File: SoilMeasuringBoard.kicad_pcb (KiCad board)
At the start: 2 copper layers, 22.5 x 100 mm, 40 parts, among them J1 USB_B_Micro, J2 BATT_CONN, J3 Conn_01x07, Q1 Q_NMOS_GSD, Q2 DMP3099L-13, Q3 DMP3099L-13, U1 RFD77101, U2 MCP73811T-420I-OT, U3 TLV74130, U4 DS18B20U, U5 SST26VF016B

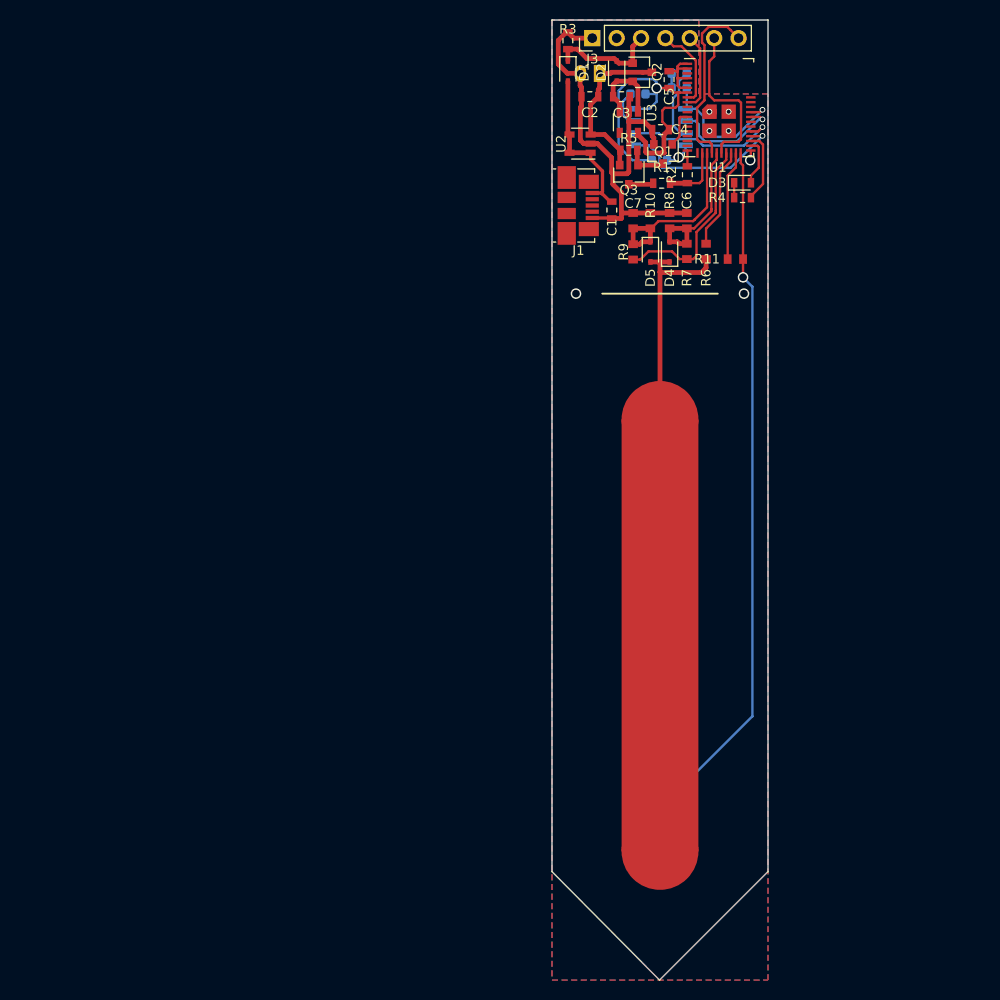
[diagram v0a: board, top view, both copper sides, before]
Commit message: final fixes
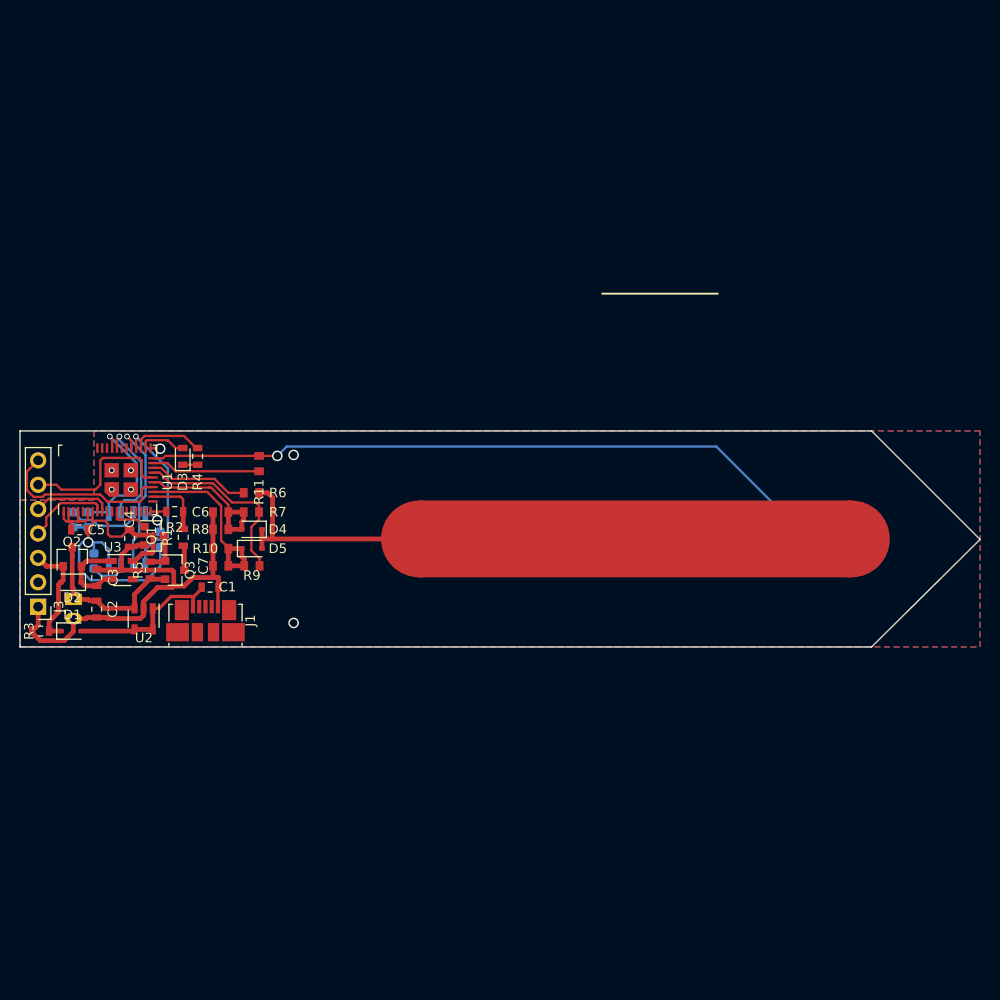
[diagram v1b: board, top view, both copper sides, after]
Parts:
- moved J3 82.7 mm to (84.1, 99.3), turned to 180 degrees
- moved R3 82.4 mm to (84.4, 101.8), turned to 180 degrees
- moved R13 78.4 mm to (87.8, 90.3), turned to 90 degrees
- moved D1 78.0 mm to (87.6, 101.8), turned to 0 degrees
- moved Q2 77.9 mm to (87.7, 94.1), turned to 90 degrees
- moved D2 77.9 mm to (87.6, 96.8), turned to 180 degrees
- moved J2 77.5 mm to (87.8, 98.5), turned to 270 degrees
- moved C5 77.3 mm to (88.4, 91.3), turned to 180 degrees
- moved R14 76.3 mm to (89.3, 90.3), turned to 90 degrees
- moved R12 74.7 mm to (89.9, 94.6), turned to 270 degrees
- moved U1 74.6 mm to (91.4, 86.1), turned to 90 degrees
- moved C3 74.1 mm to (90.2, 96.3), turned to 90 degrees
- moved C2 74.1 mm to (90.2, 99.6), turned to 270 degrees
- moved U3 70.4 mm to (92.9, 95.5), turned to 0 degrees
- moved U5 70.1 mm to (93.4, 92.3), turned to 270 degrees
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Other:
- board size 22.5 x 100 mm -> 100 x 22.5 mm
